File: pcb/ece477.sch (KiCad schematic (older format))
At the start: 10 parts, among them J1 ADA751, J2 ADA254, J3 ESP_UART, SW1 SW_Push, U1 ESP32-WROOM-32

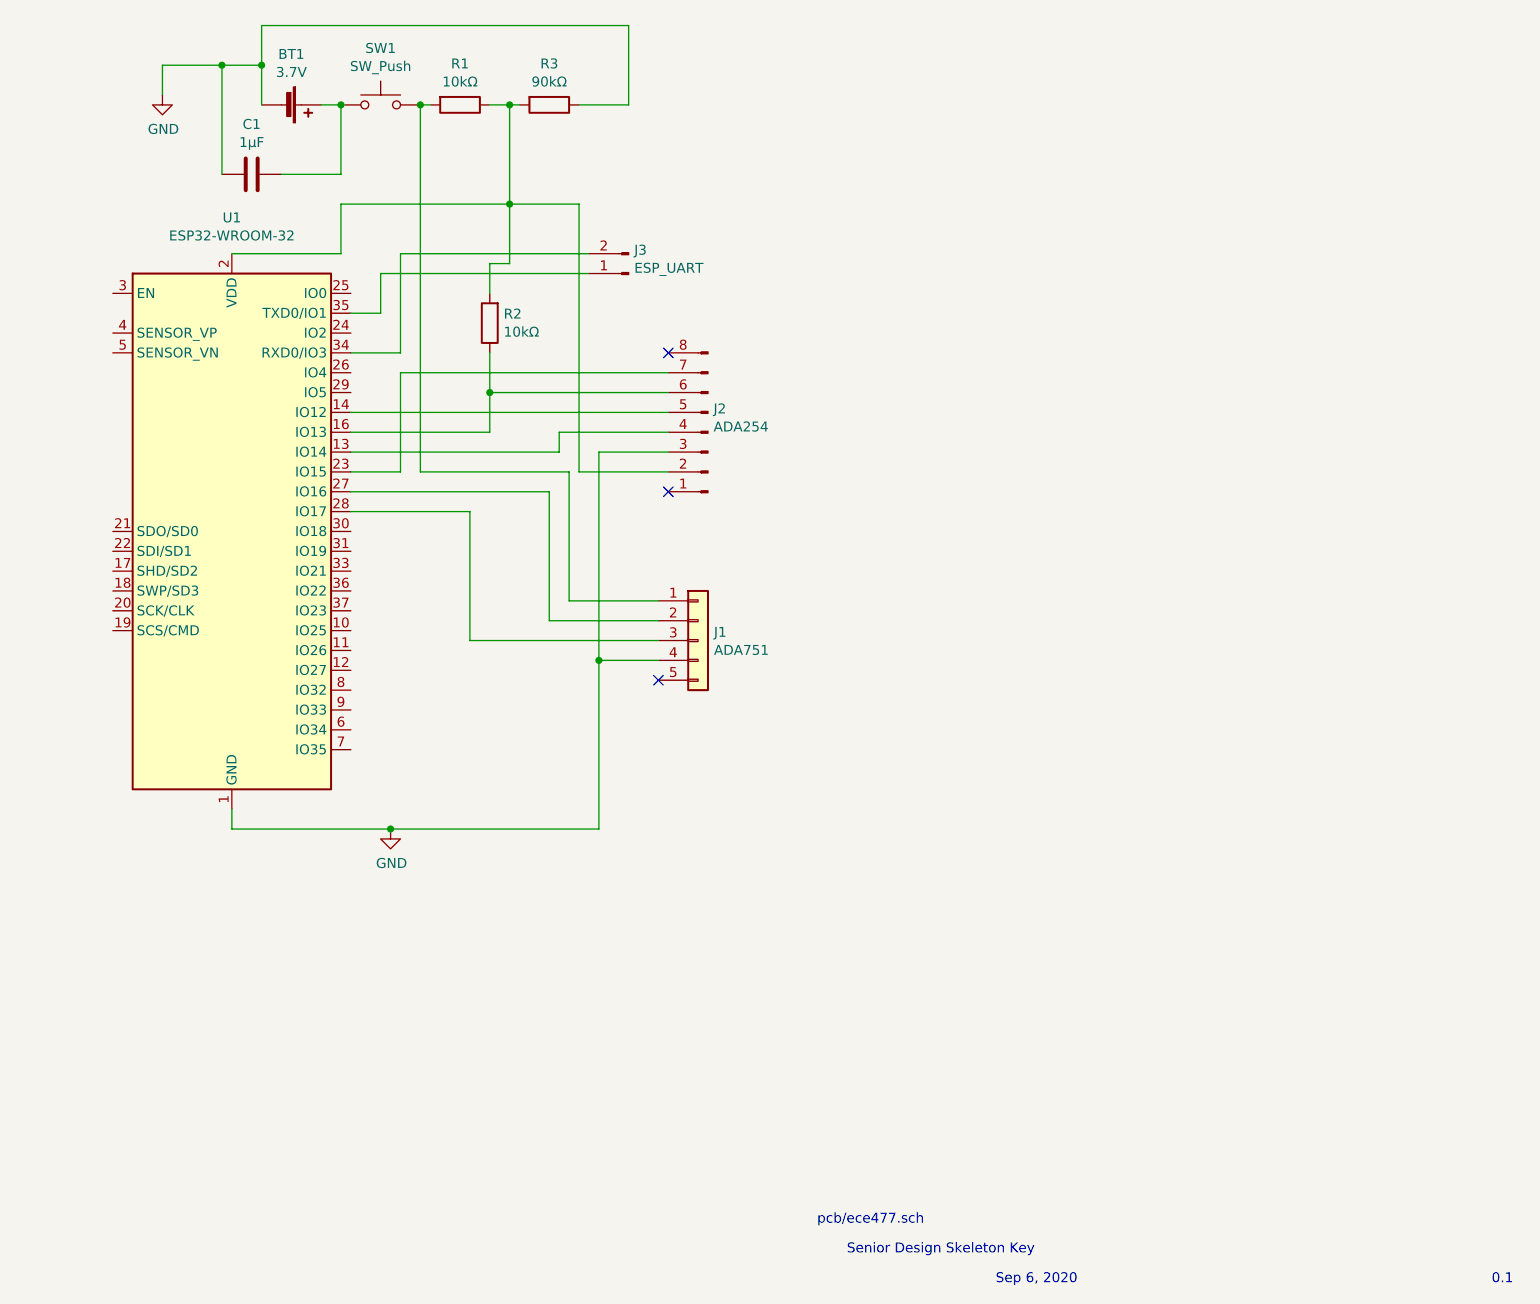
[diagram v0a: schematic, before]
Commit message: cleanup
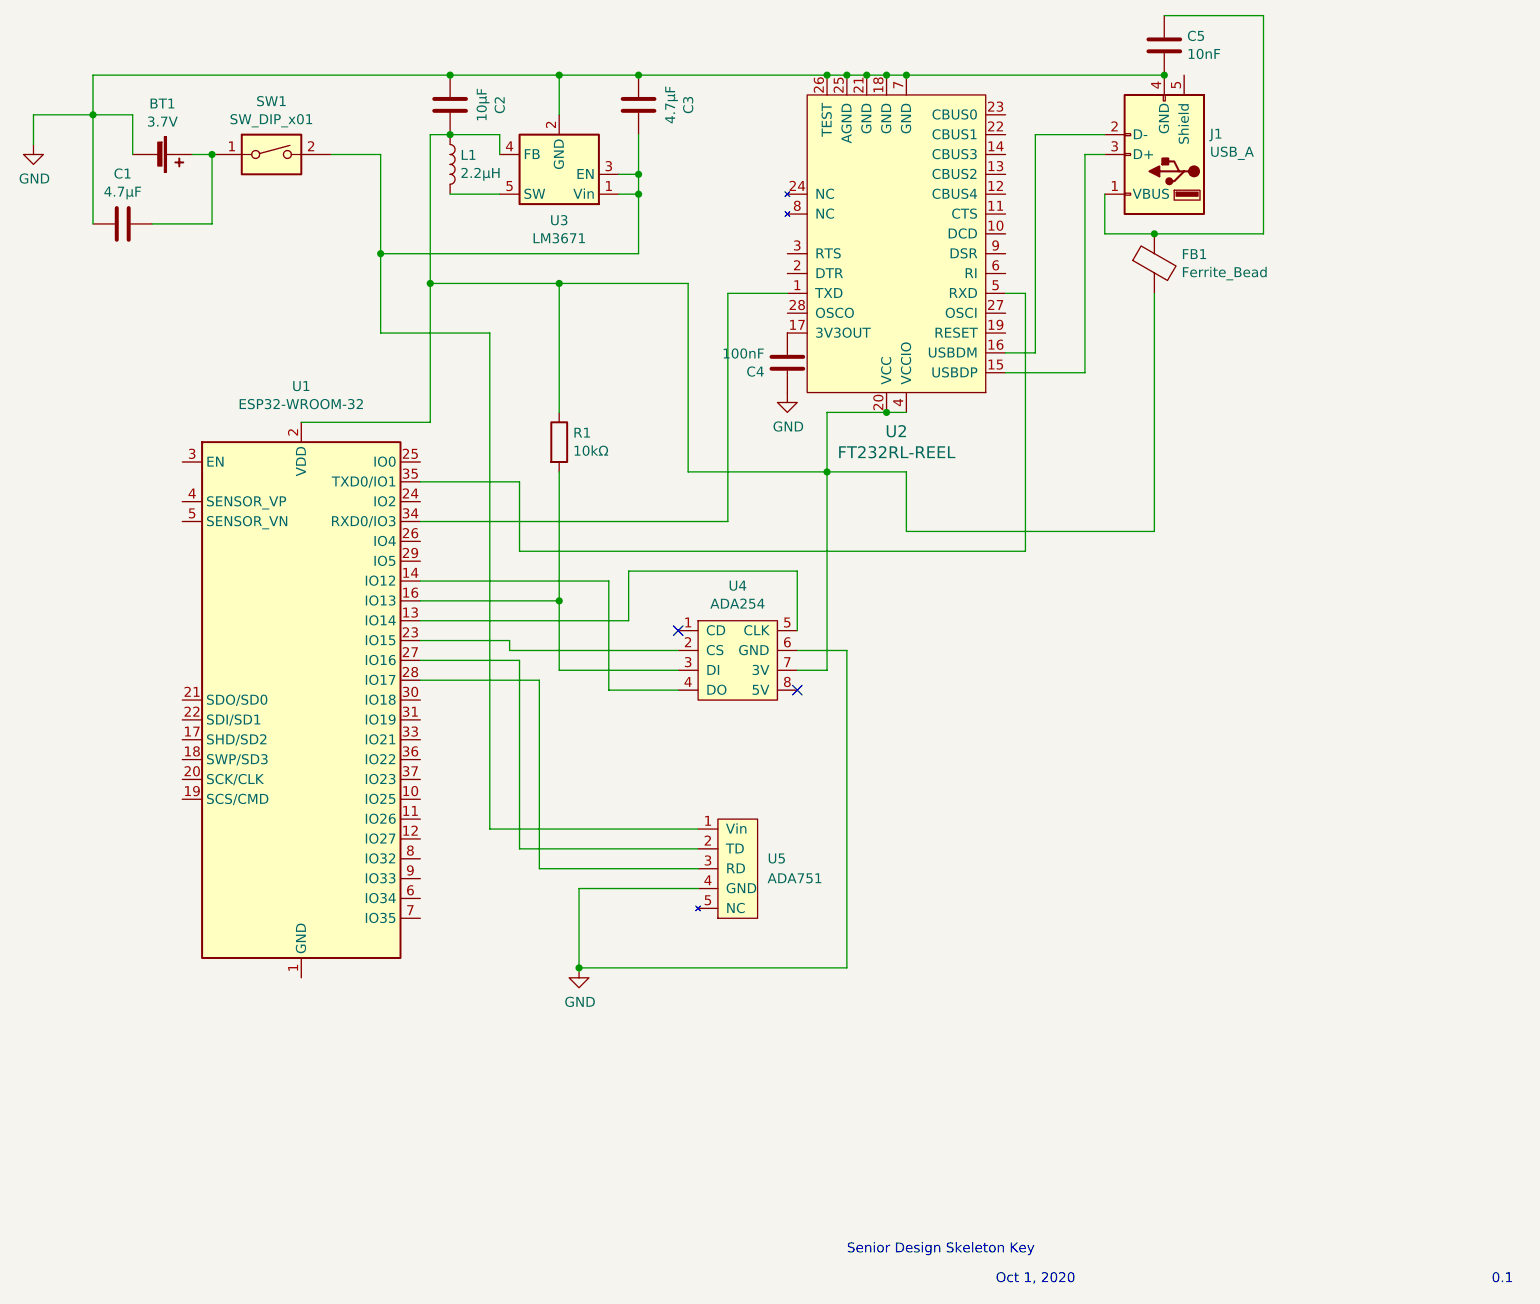
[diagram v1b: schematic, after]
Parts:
- removed J1: ADA751, Connector_PinHeader_2.00mm:PinHeader_1x05_P2.00mm_Vertical, symbol Connector_Generic:Conn_01x05
- removed J2: ADA254, Connector_PinHeader_2.00mm:PinHeader_1x08_P2.00mm_Vertical, symbol Connector:Conn_01x08_Male
- removed J3: ESP_UART, Connector_PinHeader_2.00mm:PinHeader_1x02_P2.00mm_Vertical, symbol Connector:Conn_01x02_Male
- removed R2: 10kΩ, Resistor_SMD:R_0201_0603Metric, symbol Device:R
- removed R3: 90kΩ, Resistor_SMD:R_0201_0603Metric, symbol Device:R
- removed SW1: SW_Push, Button_Switch_SMD:SW_DIP_SPSTx01_Slide_6.7x4.1mm_W6.73mm_P2.54mm_LowProfile_JPin, symbol Switch:SW_Push
- added C2: 10µF, Capacitor_SMD:CP_Elec_3x5.3, symbol Device:C
- added C3: 4.7µF, Capacitor_SMD:CP_Elec_3x5.3, symbol Device:C
- added C4: 100nF, Capacitor_SMD:CP_Elec_3x5.3, symbol Device:C
- added C5: 10nF, Capacitor_SMD:CP_Elec_3x5.3, symbol Device:C
- added FB1: Ferrite_Bead, Ferrite_THT:LairdTech_28C0236-0JW-10, symbol Device:Ferrite_Bead
- added J1: USB_A, digikey-footprints:USB_Male_A_UP2-AH-1-TH, symbol Connector:USB_A
- added L1: 2.2µH, Inductor_SMD:L_7.3x7.3_H4.5, symbol Device:L
- added SW1: SW_DIP_x01, Button_Switch_SMD:SW_DIP_SPSTx01_Slide_6.7x4.1mm_W6.73mm_P2.54mm_LowProfile_JPin, symbol Switch:SW_DIP_x01
- added U2: FT232RL-REEL, digikey-footprints:SSOP-28_W5.30mm, symbol dk_Interface-Controllers:FT232RL-REEL
- added U3: LM3671, Package_TO_SOT_SMD:TSOT-23-5, symbol Regulator_Switching:LM3670MF
- added U4: ADA254, Connector_PinSocket_2.00mm:PinSocket_1x08_P2.00mm_Vertical, symbol Device:ADA254
- added U5: ADA751, Connector_PinHeader_2.00mm:PinHeader_1x05_P2.00mm_Vertical, symbol Device:ADA751
- BT1: footprint Connector_PinHeader_2.00mm:PinHeader_1x02_P2.00mm_Vertical -> Button_Switch_SMD:SW_DIP_SPSTx01_Slide_6.7x4.1mm_W6.73mm_P2.54mm_LowProfile_JPin
- C1: value 1µF -> 4.7µF
- U1: footprint Package_DFN_QFN:QFN-48-1EP_5x5mm_P0.35mm_EP3.7x3.7mm -> digikey-footprints:ESP32-WROOM-32D
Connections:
- net GND: now also C2.1, C3.1, C4.1, C5.2, J1.4 (GND), U2.18 (GND), U2.21 (GND), U2.25 (AGND), U2.26 (TEST), U2.7 (GND), U3.2 (GND), U4.6 (GND), U5.4 (GND); no longer U1.1 (GND), U1.15 (GND), U1.38 (GND), U1.39 (GND)
- net at U1.13 (IO14): now also U4.5 (CLK)
- net at U1.14 (IO12): now also U4.4 (DO)
- net at U1.16 (IO13): now also R1.2, U4.3 (DI)
- net at R1.1, U1.2 (VDD): now also C2.2, FB1.2, L1.1, U2.20 (VCC), U2.4 (VCCIO), U3.4 (FB), U4.7 (3V)
- net at U1.23 (IO15): now also U4.2 (CS)
- net at U1.27 (IO16): now also U5.2 (TD)
- net at U1.28 (IO17): now also U5.3 (RD)
- net at U1.34 (RXD0/IO3): now also U2.1 (TXD)
- net at U1.35 (TXD0/IO1): now also U2.5 (RXD)
- net at BT1.1 (+), C1.2: now also SW1.1
- new net: U1.1 (GND), U1.15 (GND), U1.38 (GND), U1.39 (GND)
- new net: C3.2, SW1.2, U3.1 (Vin), U3.3 (EN), U5.1 (Vin)
- new net: C4.2, U2.17 (3V3OUT)
- new net: C5.1, FB1.1, J1.1 (VBUS)
- new net: J1.2 (D-), U2.16 (USBDM)
- new net: J1.3 (D+), U2.15 (USBDP)
- new net: L1.2, U3.5 (SW)
- no-connect marks 3 -> 2
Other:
- note added: "Oct 1, 2020"
- note removed: "Sep 6, 2020"
- note removed: "pcb/ece477.sch"
- moved on the sheet: BT1, C1, U1
